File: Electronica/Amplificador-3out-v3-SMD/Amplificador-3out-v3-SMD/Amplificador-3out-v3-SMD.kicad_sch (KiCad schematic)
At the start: 32 parts, among them Q1 MPF102, SW1 SW_DPST_x2, SW2 SW_DPST_x2, U1 LM386

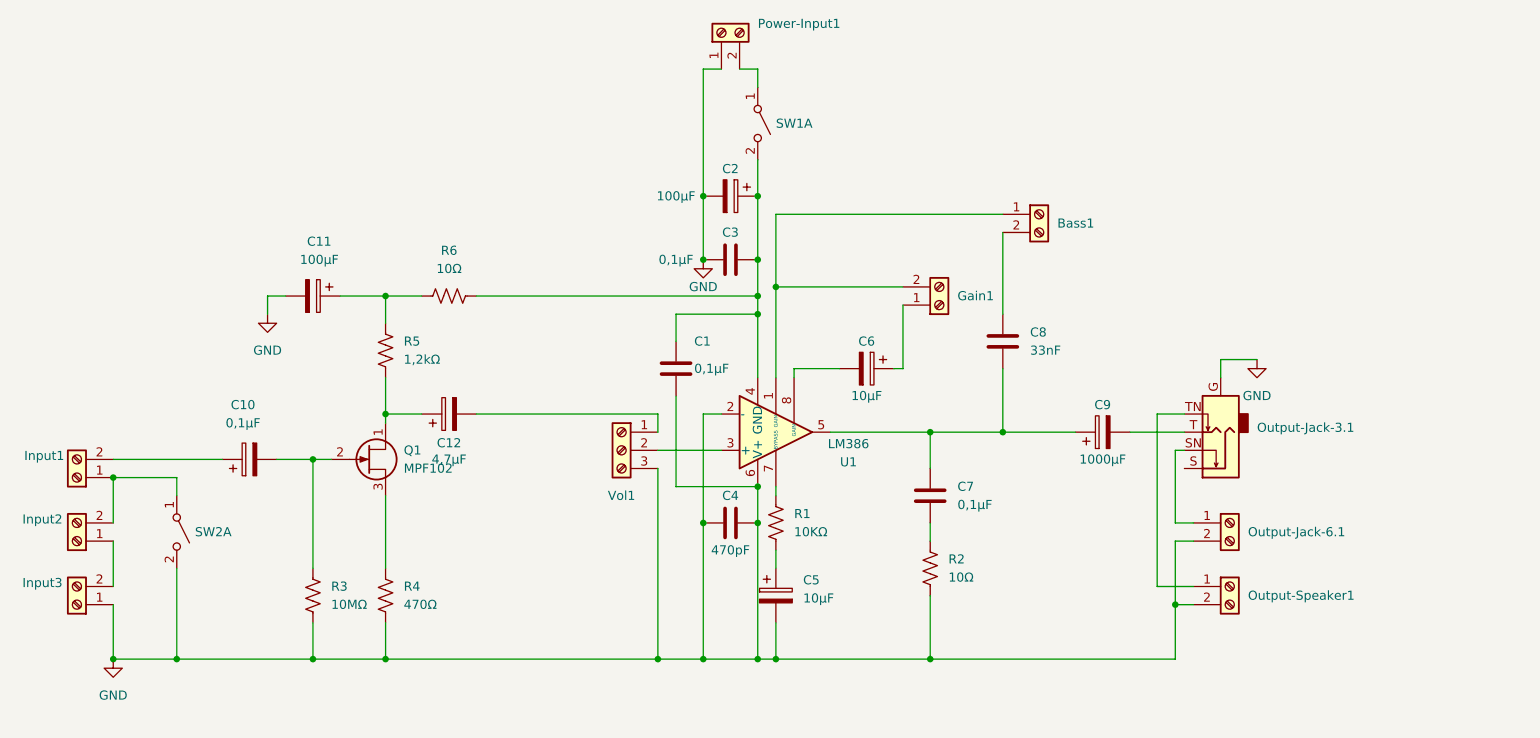
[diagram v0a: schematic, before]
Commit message: Amp v2 sin plano masa
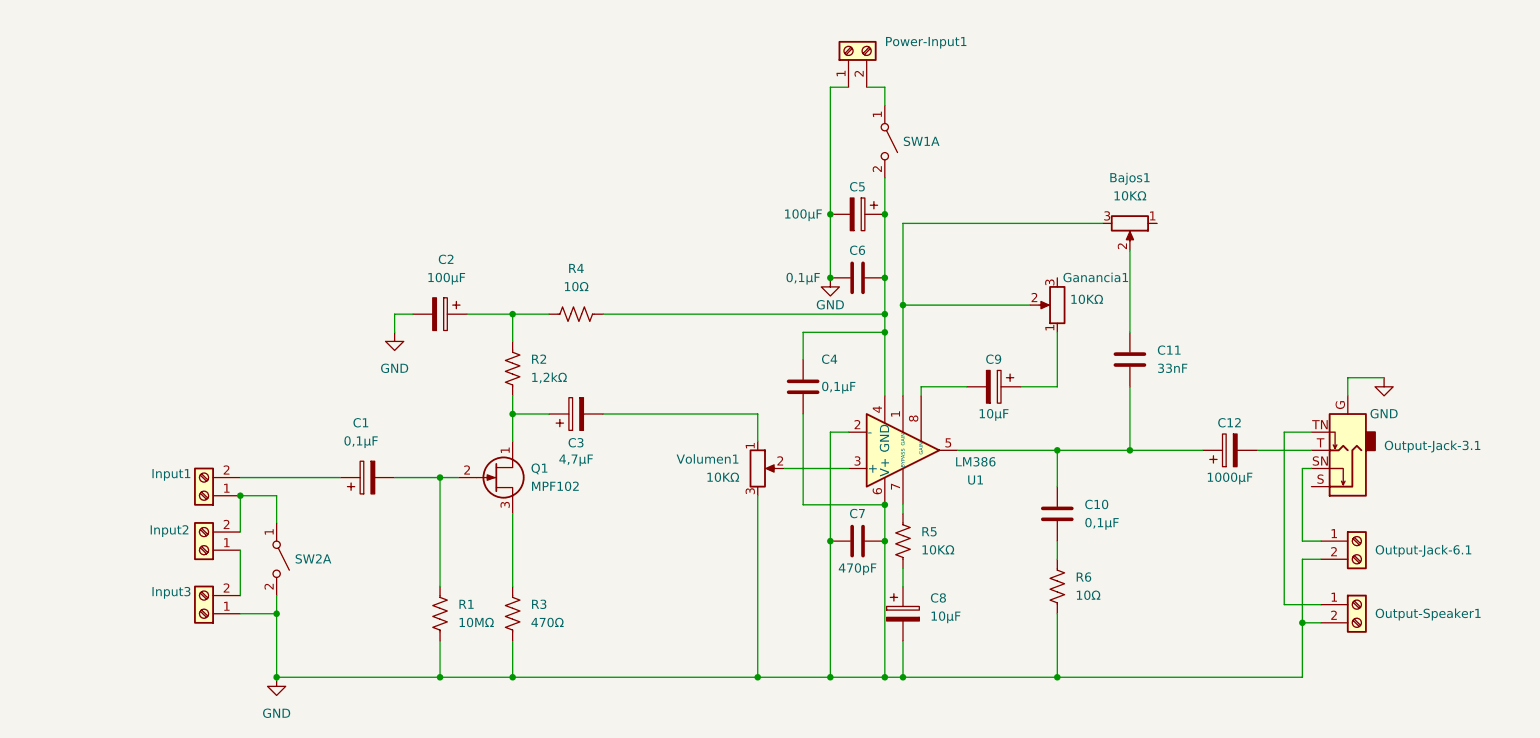
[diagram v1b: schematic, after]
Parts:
- removed Bass1, Gain1: Screw_Terminal_01x02, Connector_Molex:Molex_KK-254_AE-6410-02A_1x02_P2.54mm_Vertical, symbol Connector:Screw_Terminal_01x02
- removed C1, C3: 0,1µF, Capacitor_THT:C_Disc_D5.0mm_W2.5mm_P2.50mm, symbol Device:C
- removed C10: 0,1µF, Capacitor_THT:CP_Radial_D6.3mm_P2.50mm, symbol Device:C_Polarized
- removed C11: 100µF, Capacitor_THT:CP_Radial_D5.0mm_P2.50mm, symbol Device:C_Polarized
- removed C6: 10µF, Capacitor_THT:CP_Radial_D4.0mm_P1.50mm, symbol Device:C_Polarized
- removed C8: 33nF, Capacitor_THT:C_Disc_D5.0mm_W2.5mm_P2.50mm, symbol Device:C
- removed Vol1: Screw_Terminal_01x03, Connector_Molex:Molex_KK-254_AE-6410-03A_1x03_P2.54mm_Vertical, symbol Connector:Screw_Terminal_01x03
- added Bajos1, Ganancia1, Volumen1: 10KΩ, Connector_Molex:Molex_KK-254_AE-6410-03A_1x03_P2.54mm_Vertical, symbol Device:R_Potentiometer
- added C1: 0,1µF, Capacitor_SMD:CP_Elec_3x5.3, symbol Device:C_Polarized
- added C10, C6: 0,1µF, Capacitor_SMD:C_0201_0603Metric, symbol Device:C
- added C11: 33nF, Capacitor_SMD:C_0201_0603Metric, symbol Device:C
- added C3: 4,7µF, Capacitor_SMD:CP_Elec_3x5.3, symbol Device:C_Polarized
- added C8: 10µF, Capacitor_SMD:CP_Elec_3x5.3, symbol Device:C_Polarized
- C12: value 4,7µF -> 1000µF; footprint Capacitor_THT:CP_Radial_D4.0mm_P1.50mm -> Capacitor_SMD:CP_Elec_3x5.3
- C2: footprint Capacitor_THT:CP_Radial_D5.0mm_P2.50mm -> Capacitor_SMD:CP_Elec_3x5.3
- C4: value 470pF -> 0,1µF; footprint Capacitor_THT:C_Disc_D5.0mm_W2.5mm_P2.50mm -> Capacitor_SMD:C_0201_0603Metric
- C5: value 10µF -> 100µF; footprint Capacitor_THT:CP_Radial_D4.0mm_P1.50mm -> Capacitor_SMD:CP_Elec_3x5.3
- C7: value 0,1µF -> 470pF; footprint Capacitor_THT:C_Disc_D5.0mm_W2.5mm_P2.50mm -> Capacitor_SMD:C_0201_0603Metric
- C9: value 1000µF -> 10µF; footprint Capacitor_THT:CP_Radial_Tantal_D9.0mm_P5.00mm -> Capacitor_SMD:CP_Elec_3x5.3
- R1: value 10KΩ -> 10MΩ; footprint Resistor_THT:R_Axial_DIN0204_L3.6mm_D1.6mm_P7.62mm_Horizontal -> Resistor_SMD:R_0201_0603Metric
- R2: value 10Ω -> 1,2kΩ; footprint Resistor_THT:R_Axial_DIN0204_L3.6mm_D1.6mm_P7.62mm_Horizontal -> Resistor_SMD:R_0201_0603Metric
- R3: value 10MΩ -> 470Ω; footprint Resistor_THT:R_Axial_DIN0204_L3.6mm_D1.6mm_P7.62mm_Horizontal -> Resistor_SMD:R_0201_0603Metric
- R4: value 470Ω -> 10Ω
- R5: value 1,2kΩ -> 10KΩ; footprint Resistor_THT:R_Axial_DIN0204_L3.6mm_D1.6mm_P7.62mm_Horizontal -> Resistor_SMD:R_0201_0603Metric
- R6: footprint Resistor_THT:R_Axial_DIN0204_L3.6mm_D1.6mm_P7.62mm_Horizontal -> Resistor_SMD:R_0201_0603Metric
- SW2: footprint Button_Switch_THT:SW_Slide_SPDT_Straight_CK_OS102011MS2Q -> Button_Switch_SMD:SW_DIP_SPSTx01_Slide_6.7x4.1mm_W6.73mm_P2.54mm_LowProfile_JPin
- U1: footprint Package_DIP:DIP-8_W7.62mm_LongPads -> Package_DIP:DIP-8_W7.62mm_SMDSocket_SmallPads
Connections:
- net GND: now also C7.1, C7.2, R1.2, R6.2, C6.1, C8.2, Volumen1.3; no longer C4.1, R2.2, R4.2
- net at Input1.2 (Pin_2): now also C1.1
- net at Q1.2 (G): now also R1.1, C1.2; no longer R3.1
- net at SW1.2 (B), U1.4 (GND): now also C4.1, C5.1, R4.2, C6.2; no longer C2.1, R6.2
- net at U1.7 (BYPASS): now also R5.1; no longer R1.1
- net at R4.1: now also C2.1, R2.1; no longer Q1.3 (S)
- net at U1.1 (GAIN): now also Bajos1.3, Ganancia1.2
- net at C12.2: now also Output-Jack-3.1.T
- net at U1.3 (+): now also Volumen1.2
- net at C9.2: now also U1.8 (GAIN); no longer Output-Jack-3.1.T
- net at R6.1: now also C10.2; no longer R5.1
- new net: C3.1, Q1.1 (D), R2.2
- new net: C10.1, C11.2, C12.1, U1.5
- new net: C9.1, Ganancia1.1
- new net: Bajos1.2, C11.1
- new net: Q1.3 (S), R3.1
- new net: C8.1, R5.2
- new net: C3.2, Volumen1.1
